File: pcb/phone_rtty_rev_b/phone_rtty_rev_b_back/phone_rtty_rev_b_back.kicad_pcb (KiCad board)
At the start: 2 copper layers, 58 x 24 mm, 3 parts

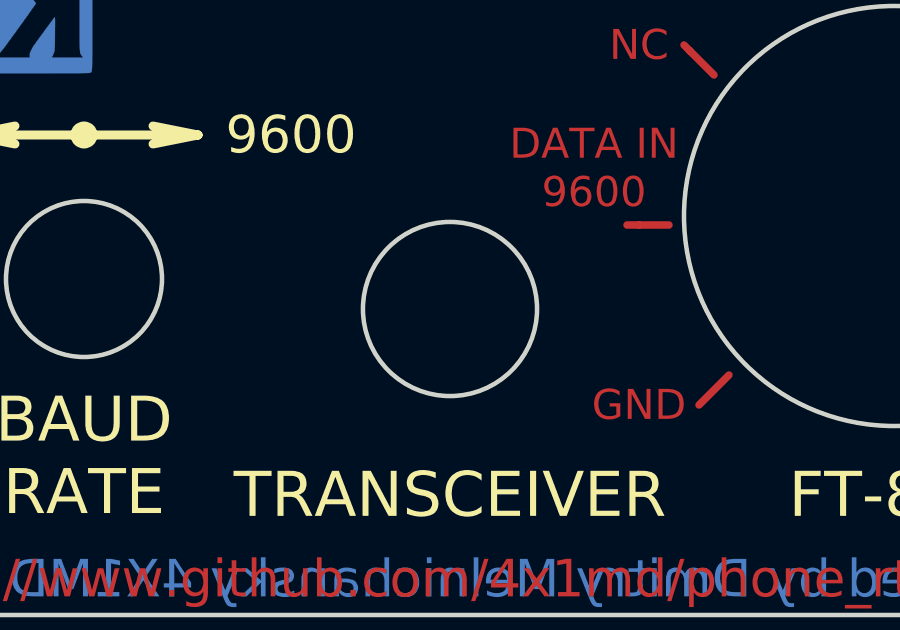
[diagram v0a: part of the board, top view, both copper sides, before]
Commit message: Minor changes.
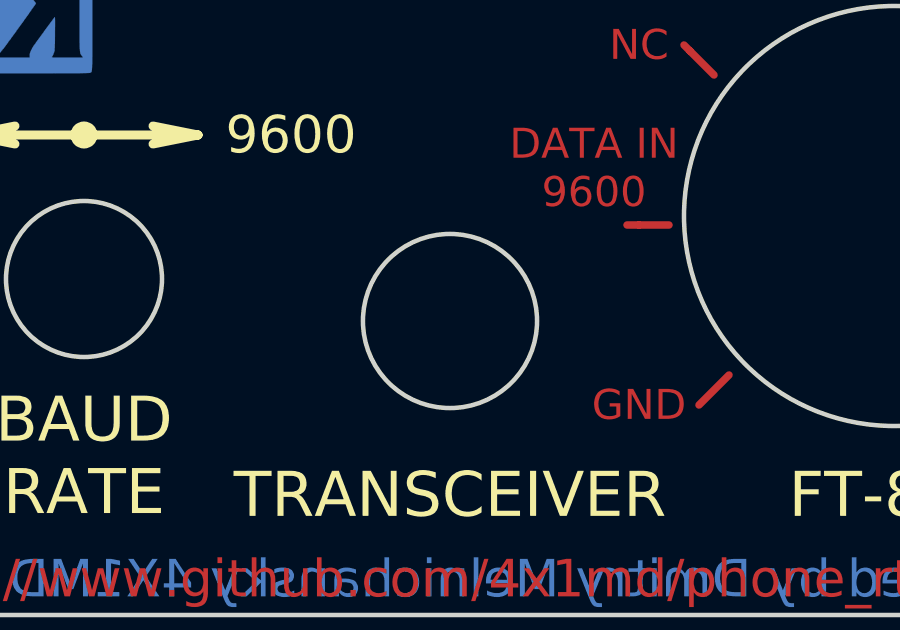
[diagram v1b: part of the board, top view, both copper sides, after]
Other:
- outline, holes or cut-outs redrawn
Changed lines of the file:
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@@
     (links 0)
     (no_connects 0)
-    (area 99.924999 99.924999 158.075001 124.075001)
+    (area 78.816667 85.65 164.986666 141.700001)
     (thickness 1.6)
     (drawings 49)
@@
   (gr_line (start 110.4 112.8) (end 116.6 112.8) (angle 90) (layer Dwgs.User) (width 0.05))
   (gr_line (start 113.5 109.7) (end 113.5 115.9) (angle 90) (layer Dwgs.User) (width 0.05))
-  (gr_line (start 125.7 110.4) (end 125.7 117.2) (angle 90) (layer Dwgs.User) (width 0.05))
-  (gr_line (start 121.8 113.8) (end 129.6 113.8) (angle 90) (layer Dwgs.User) (width 0.05))
+  (gr_line (start 125.7 110.8) (end 125.7 117.6) (angle 90) (layer Dwgs.User) (width 0.05))
+  (gr_line (start 121.8 114.2) (end 129.6 114.2) (angle 90) (layer Dwgs.User) (width 0.05))
   (gr_text "PCB level" (at 105 116) (layer Cmts.User)
     (effects (font (size 1.2 1.2) (thickness 0.1)))
@@
     (effects (font (size 1.5 1.5) (thickness 0.3)))
   )
-  (gr_circle (center 125.7 113.8) (end 128.6 113.7) (layer Edge.Cuts) (width 0.15))
+  (gr_circle (center 125.7 114.2) (end 128.6 114.1) (layer Edge.Cuts) (width 0.15))
   (gr_line (start 100 116.7) (end 158 116.7) (angle 90) (layer Dwgs.User) (width 0.05))
   (gr_arc (start 101 101) (end 100 101) (angle 90) (layer Edge.Cuts) (width 0.15))

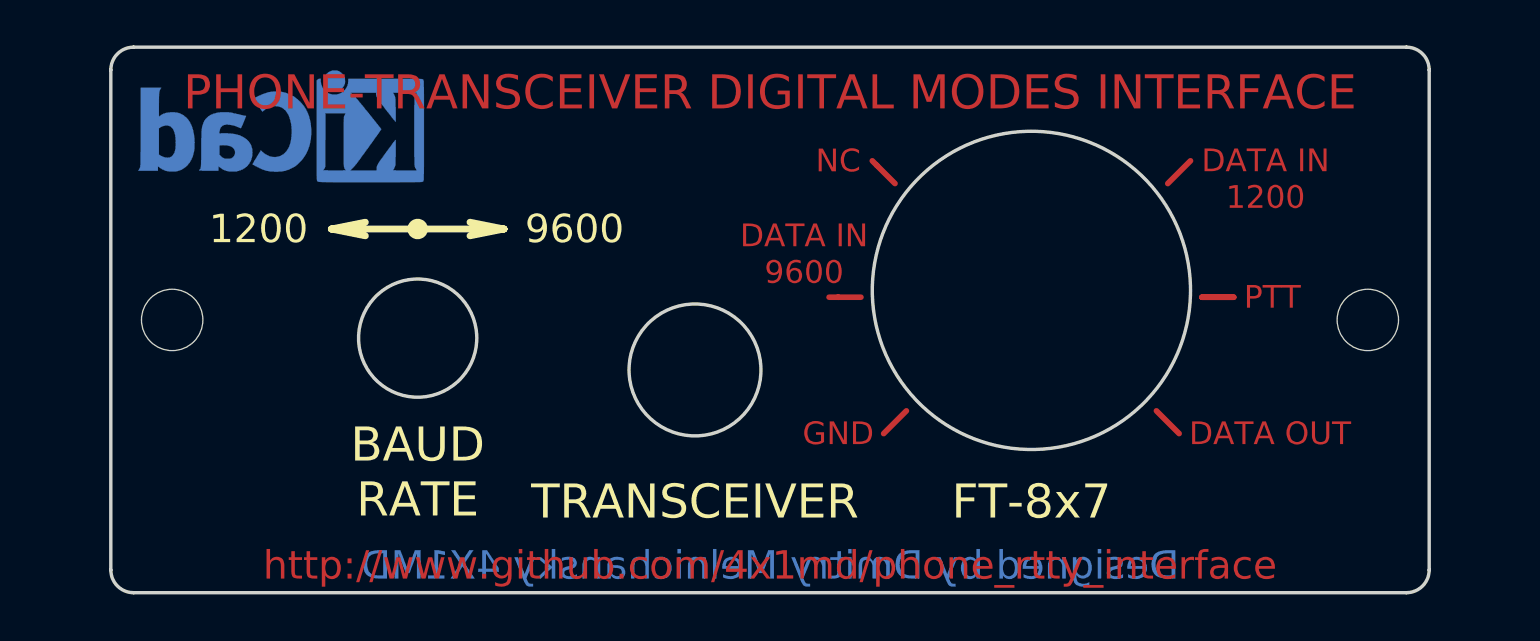
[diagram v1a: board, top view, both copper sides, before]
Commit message: Minor changes to revision B and gerbers.
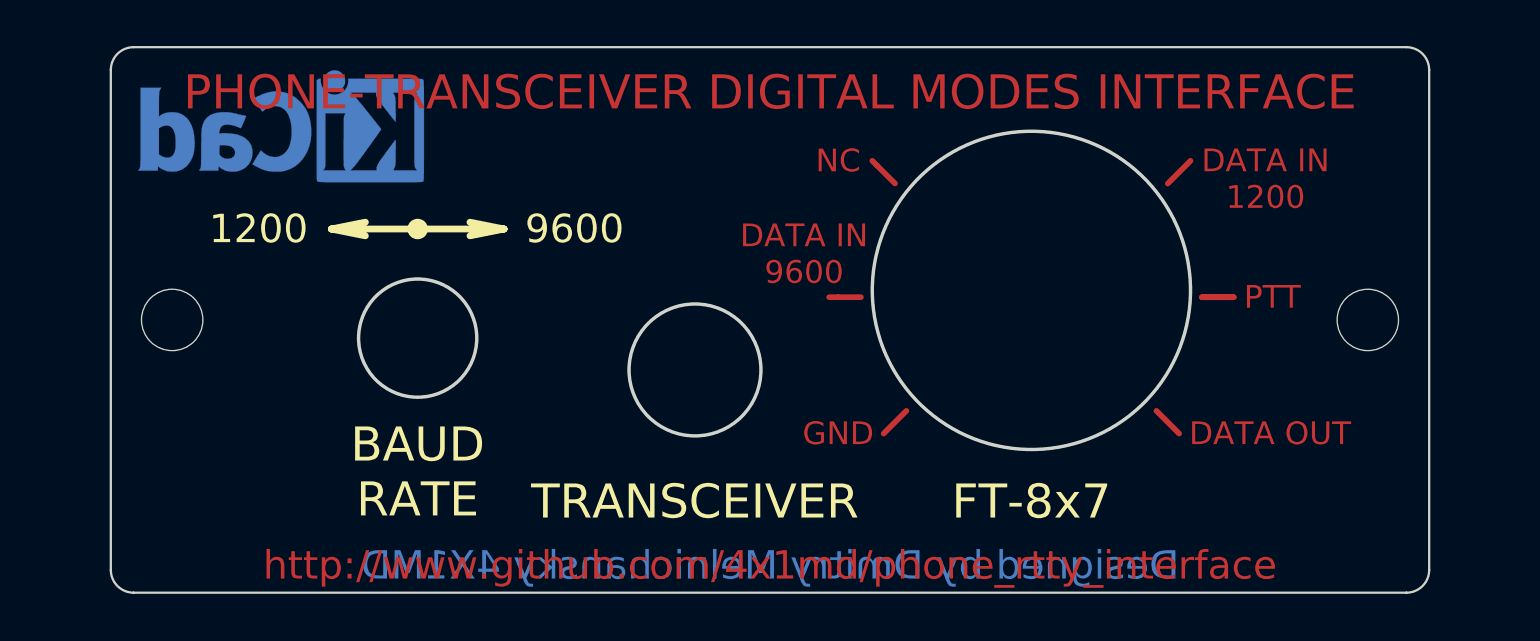
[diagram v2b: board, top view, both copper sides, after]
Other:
- board text added: "RTTY Interface Rev. B Back Panel"
- board text removed: "RTTY Interface Revision B Back Panel"
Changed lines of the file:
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@@
     (links 0)
     (no_connects 0)
-    (area 78.816667 85.65 164.986666 141.700001)
+    (area 78.816667 88.8 164.986666 141.700001)
     (thickness 1.6)
     (drawings 49)
@@
     (visible_elements 7FFFFFFF)
     (pcbplotparams
-      (layerselection 0x010f0_80000001)
+      (layerselection 0x010e0_80000001)
       (usegerberextensions true)
       (excludeedgelayer true)
@@
       (drillshape 0)
       (scaleselection 1)
-      (outputdirectory D:/MyProjects/phone_rtty_interface/gerbers))
+      (outputdirectory gerbers))
   )
   (net 0 "")
@@
   (gr_circle (center 125.7 114.2) (end 128.6 114.1) (layer Edge.Cuts) (width 0.15))
   (gr_line (start 100 116.7) (end 158 116.7) (angle 90) (layer Dwgs.User) (width 0.05))
-  (gr_arc (start 101 101) (end 100 101) (angle 90) (layer Edge.Cuts) (width 0.15))
-  (gr_arc (start 101 123) (end 101 124) (angle 90) (layer Edge.Cuts) (width 0.15))
-  (gr_arc (start 157 123) (end 158 123) (angle 90) (layer Edge.Cuts) (width 0.15))
-  (gr_arc (start 157 101) (end 157 100) (angle 90) (layer Edge.Cuts) (width 0.15))
-  (gr_text "RTTY Interface\nRevision B\nBack Panel" (at 129 90.5) (layer Cmts.User)
+  (gr_arc (start 101 101) (end 100 101) (angle 90) (layer Edge.Cuts) (width 0.1))
+  (gr_arc (start 101 123) (end 101 124) (angle 90) (layer Edge.Cuts) (width 0.1))
+  (gr_arc (start 157 123) (end 158 123) (angle 90) (layer Edge.Cuts) (width 0.1))
+  (gr_arc (start 157 101) (end 157 100) (angle 90) (layer Edge.Cuts) (width 0.1))
+  (gr_text "RTTY Interface Rev. B\nBack Panel" (at 129 92) (layer Cmts.User)
     (effects (font (size 2 2) (thickness 0.3)))
   )
@@
     (effects (font (size 1.5 1.5) (thickness 0.25)))
   )
-  (gr_line (start 158 101) (end 158 123) (angle 90) (layer Edge.Cuts) (width 0.15))
-  (gr_line (start 100 101) (end 100 123) (angle 90) (layer Edge.Cuts) (width 0.15))
-  (gr_line (start 101 100) (end 157 100) (angle 90) (layer Edge.Cuts) (width 0.15))
-  (gr_line (start 101 124) (end 157 124) (angle 90) (layer Edge.Cuts) (width 0.15))
+  (gr_line (start 158 101) (end 158 123) (angle 90) (layer Edge.Cuts) (width 0.1))
+  (gr_line (start 100 101) (end 100 123) (angle 90) (layer Edge.Cuts) (width 0.1))
+  (gr_line (start 101 100) (end 157 100) (angle 90) (layer Edge.Cuts) (width 0.1))
+  (gr_line (start 101 124) (end 157 124) (angle 90) (layer Edge.Cuts) (width 0.1))
   (segment (start 133.5 105) (end 133.7 105.2) (width 0.25) (layer F.Cu) (net 0))
   (segment (start 133.7 105.2) (end 134.5 106) (width 0.25) (layer F.Cu) (net 0))
